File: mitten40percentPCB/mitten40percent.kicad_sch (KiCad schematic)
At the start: 114 parts, among them J2 I2C, J3 USB_C_Receptacle_USB2.0_16P, SW0 SW_Push, SW1 SW_Push_45deg, SW10 SW_Push_45deg, SW11 SW_Push_45deg, SW12 SW_Push_45deg, SW13 SW_Push_45deg, SW14 SW_Push_45deg, SW15 SW_Push_45deg, SW16 SW_Push_45deg, SW17 SW_Push_45deg, SW18 SW_Push_45deg, SW19 SW_Push_45deg, SW2 SW_Push_45deg, SW20 SW_Push_45deg, SW21 SW_Push_45deg, SW22 SW_Push_45deg, SW23 SW_Push_45deg, SW24 SW_Push_45deg, SW25 SW_Push_45deg, SW26 SW_Push_45deg, SW27 SW_Push_45deg, SW28 SW_Push_45deg, SW29 SW_Push_45deg, SW3 SW_Push_45deg, SW30 SW_Push_45deg, SW31 SW_Push_45deg, SW32 SW_Push_45deg, SW33 SW_Push_45deg, SW34 SW_Push_45deg, SW35 SW_Push_45deg, SW36 SW_Push_45deg, SW37 SW_Push_45deg, SW38 SW_Push_45deg, SW39 SW_Push_45deg, SW4 SW_Push_45deg, SW40 SW_Push_45deg, SW41 SW_Push_45deg, SW42 SW_Push_45deg, SW43 SW_Push_45deg, SW44 SW_Push_45deg, SW45 SW_Push_45deg, SW46 SW_Push_45deg, SW48 Joystick, SW5 SW_Push_45deg, SW6 SW_Push_45deg, SW7 SW_Push_45deg, SW8 SW_Push_45deg, SW9 SW_Push_45deg, U1 STM32F072CBT6, U2 USBLC6-2SC6, U3 XC6206PxxxMR

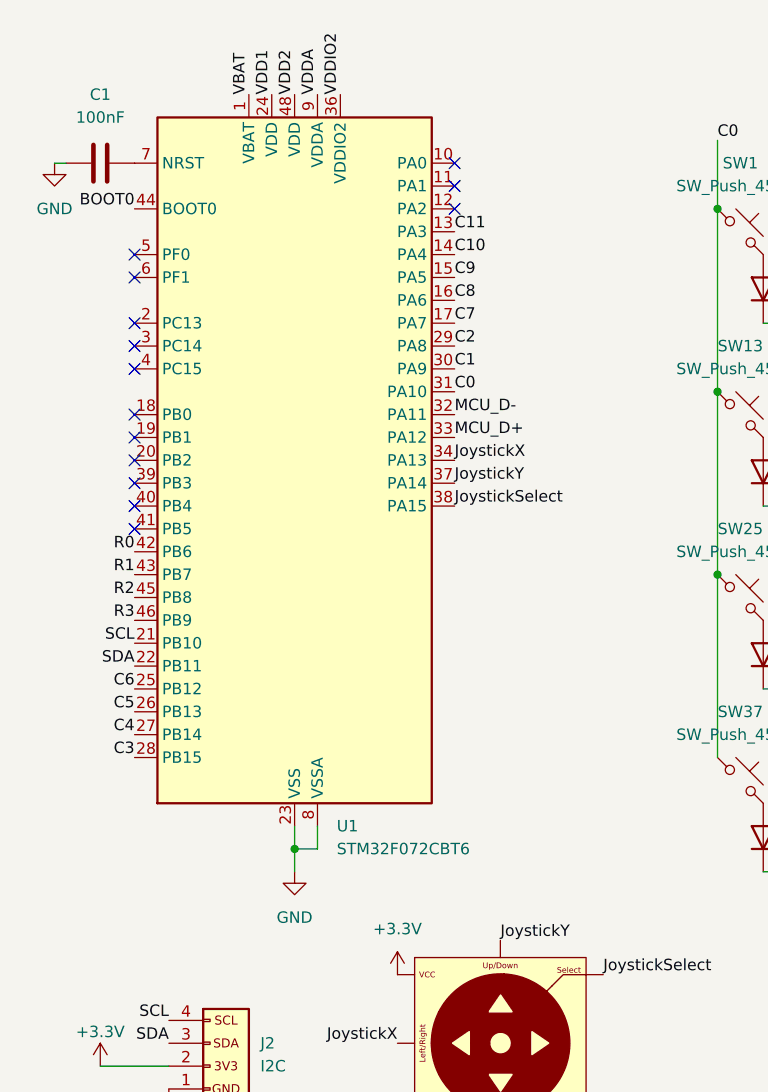
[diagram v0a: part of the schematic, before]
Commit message: finalized routing
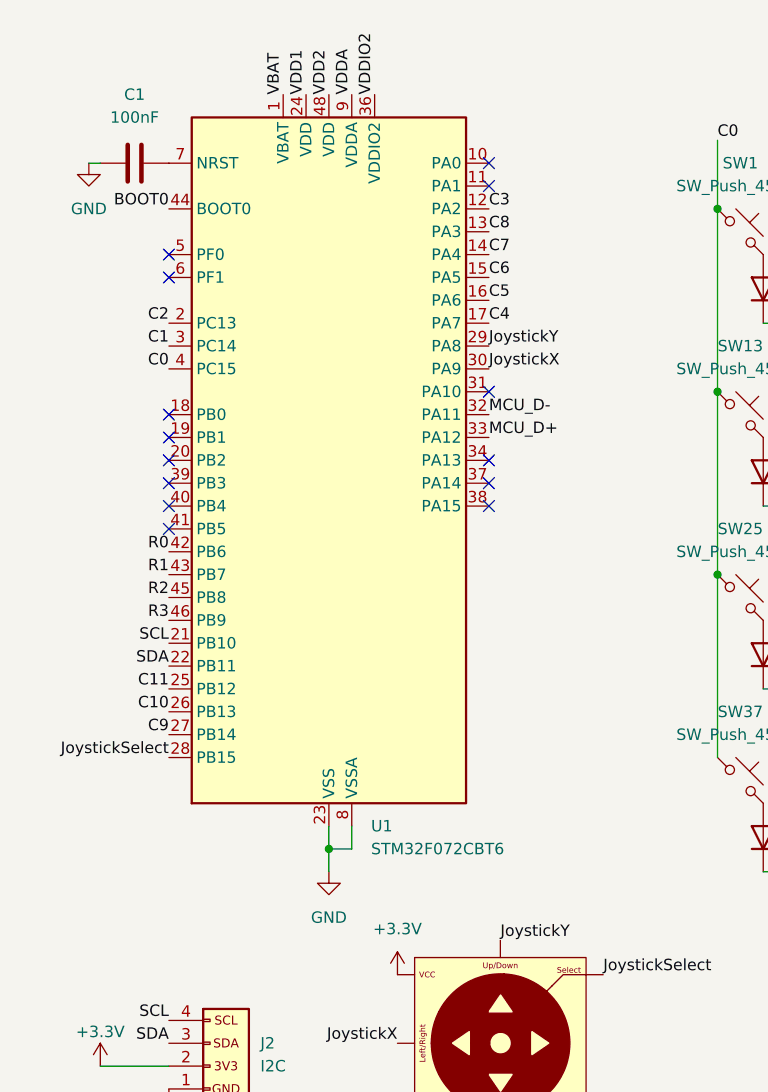
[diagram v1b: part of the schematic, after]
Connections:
- net C0: now also U1.4 (PC15); no longer U1.31 (PA10)
- net C1: now also U1.3 (PC14); no longer U1.30 (PA9)
- net C10: now also U1.26 (PB13); no longer U1.14 (PA4)
- net C11: now also U1.25 (PB12); no longer U1.13 (PA3)
- net C2: now also U1.2 (PC13); no longer U1.29 (PA8)
- net C3: now also U1.12 (PA2); no longer U1.28 (PB15)
- net C4: now also U1.17 (PA7); no longer U1.27 (PB14)
- net C5: now also U1.16 (PA6); no longer U1.26 (PB13)
- net C6: now also U1.15 (PA5); no longer U1.25 (PB12)
- net C7: now also U1.14 (PA4); no longer U1.17 (PA7)
- net C8: now also U1.13 (PA3); no longer U1.16 (PA6)
- net C9: now also U1.27 (PB14); no longer U1.15 (PA5)
- net JoystickSelect: now also U1.28 (PB15); no longer U1.38 (PA15)
- net JoystickX: now also U1.30 (PA9); no longer U1.34 (PA13)
- net JoystickY: now also U1.29 (PA8); no longer U1.37 (PA14)
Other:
- company: poo poo pee pee corporation -> bumbling idiots inc.
- moved on the sheet: C1, U1
